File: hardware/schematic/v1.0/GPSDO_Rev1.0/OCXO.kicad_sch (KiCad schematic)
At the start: 23 parts, among them U2 LMK1C1103PWR, U3 TMP117AIDRVR, U5 OCXO_20x20mm, U7 OCXO_25.4x25.4mm, U8 REF5040

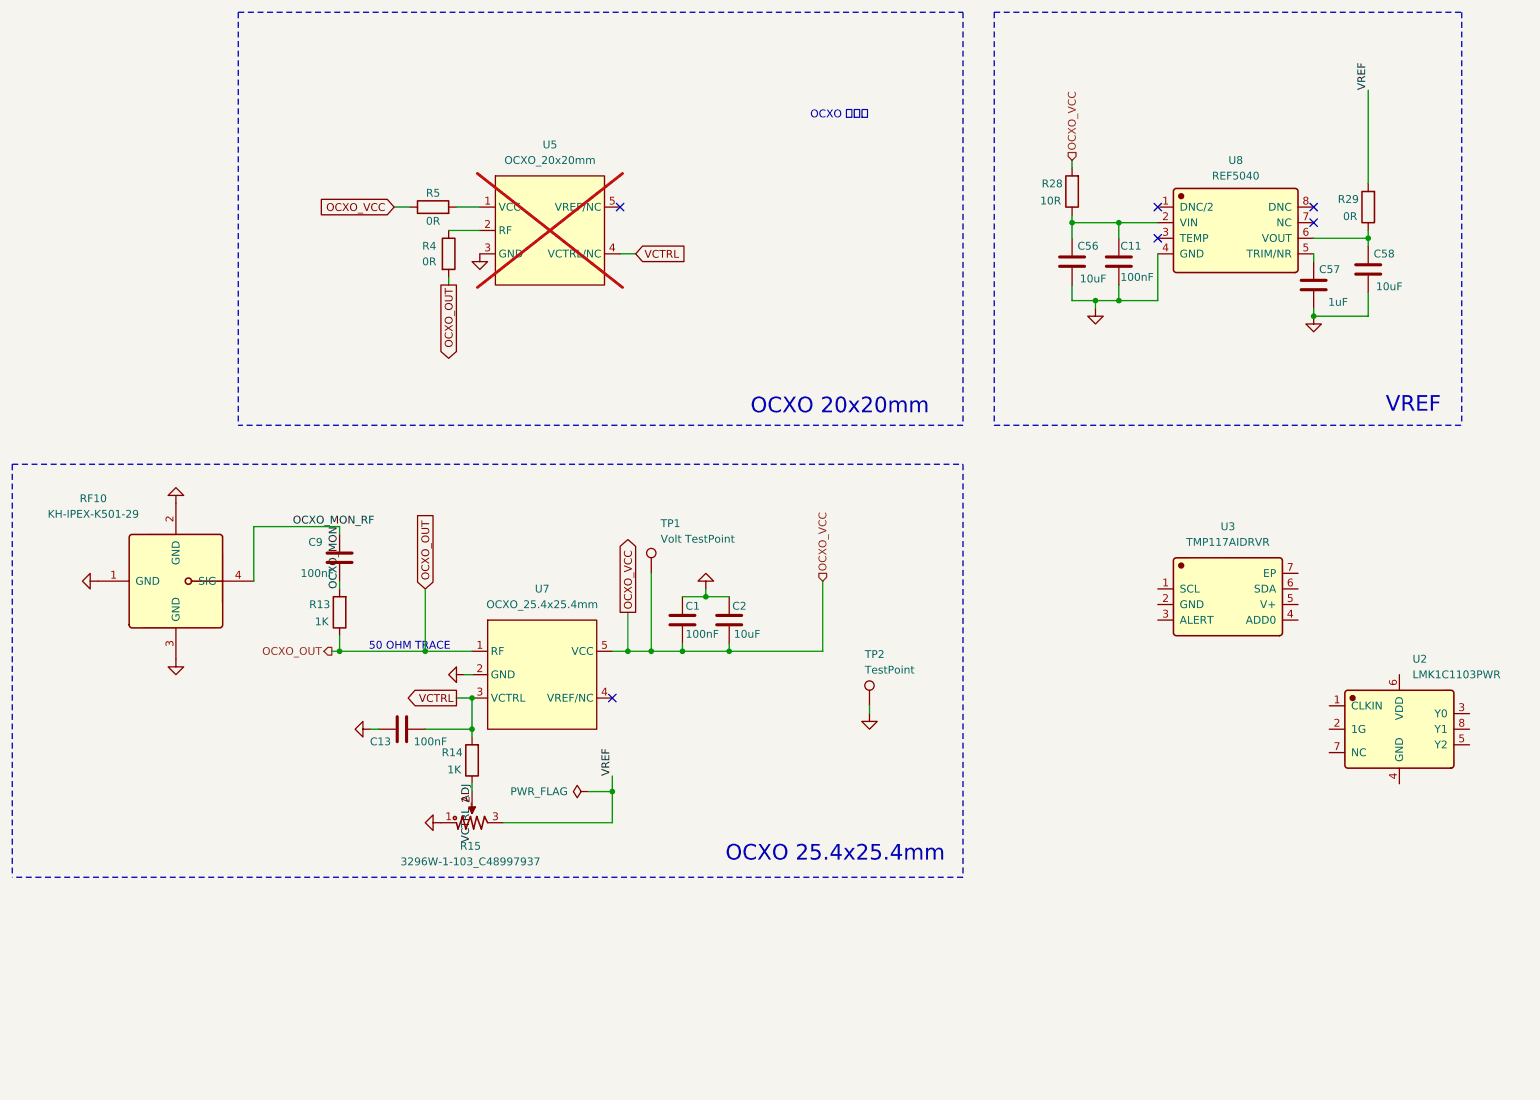
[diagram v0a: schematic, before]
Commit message: sch update
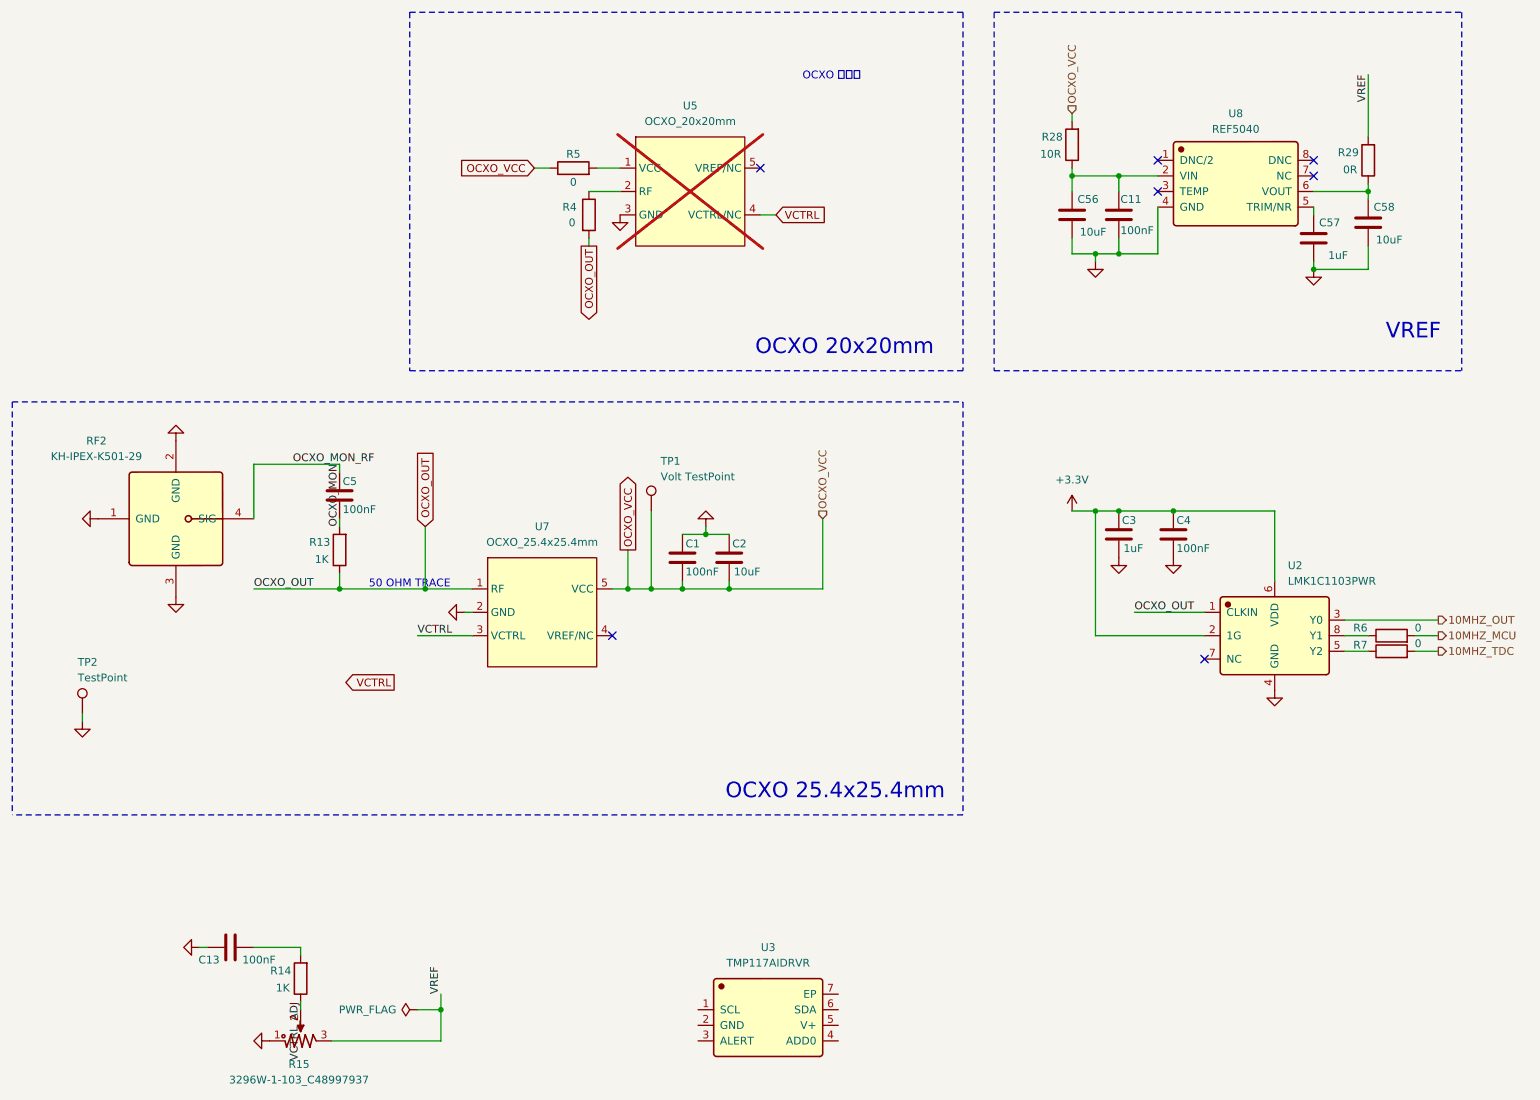
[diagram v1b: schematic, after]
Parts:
- removed C9: 100nF, Capacitor_SMD:C_0402_1005Metric, symbol Device:C
- removed RF10: KH-IPEX-K501-29, JLCImport:KH-IPEX-K501-29, symbol JLCImport:KH-IPEX-K501-29
- added C3: 1uF, GPSDO_Rev1.0:C_0603_1608Metric, symbol GPSDO_Rev1.0:C
- added C4, C5: 100nF, GPSDO_Rev1.0:C_0402_1005Metric, symbol GPSDO_Rev1.0:C
- added R6: 0, GPSDO_Rev1.0:C_0603_1608Metric, symbol GPSDO_Rev1.0:R
- added R7: 0, GPSDO_Rev1.0:R_0603_1608Metric, symbol GPSDO_Rev1.0:R
- added RF2: KH-IPEX-K501-29, GPSDO_Rev1.0:KH-IPEX-K501-29, symbol GPSDO_Rev1.0:KH-IPEX-K501-29
- R4, R5: value 0R -> 0
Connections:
- net GND: now also U2.4 (GND), C3.2, C4.2, RF2.1 (GND), RF2.2 (GND), RF2.3 (GND)
- net OCXO_MON: now also C5.2
- net OCXO_MON_RF: now also C5.1, RF2.4 (SIG)
- net OCXO_OUT: now also U2.1 (CLKIN)
- net VCTRL: no longer C13.1, R14.2
- net +3.3V: now reaches U2.2 (1G)
- net +3.3V: now also U2.6 (VDD), C3.1, C4.1
- net 10MHZ_OUT: now reaches U2.3 (Y0)
- net at U2.5 (Y2): now also R7.1
- net at U2.8 (Y1): now also R6.1
- new net: C13.1, R14.2
- new net 10MHZ_MCU: R6.2
- new net 10MHZ_TDC: R7.2
- no-connect marks 6 -> 7
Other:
- moved on the sheet: C1, C11, C2, C56, C57, C58, R13, R28, R29, R4, R5, TP1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
